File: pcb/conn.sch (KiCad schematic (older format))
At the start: 11 parts, among them P1 CONN_16X2, P2 CONN_16X2, P3 CONN_5X2

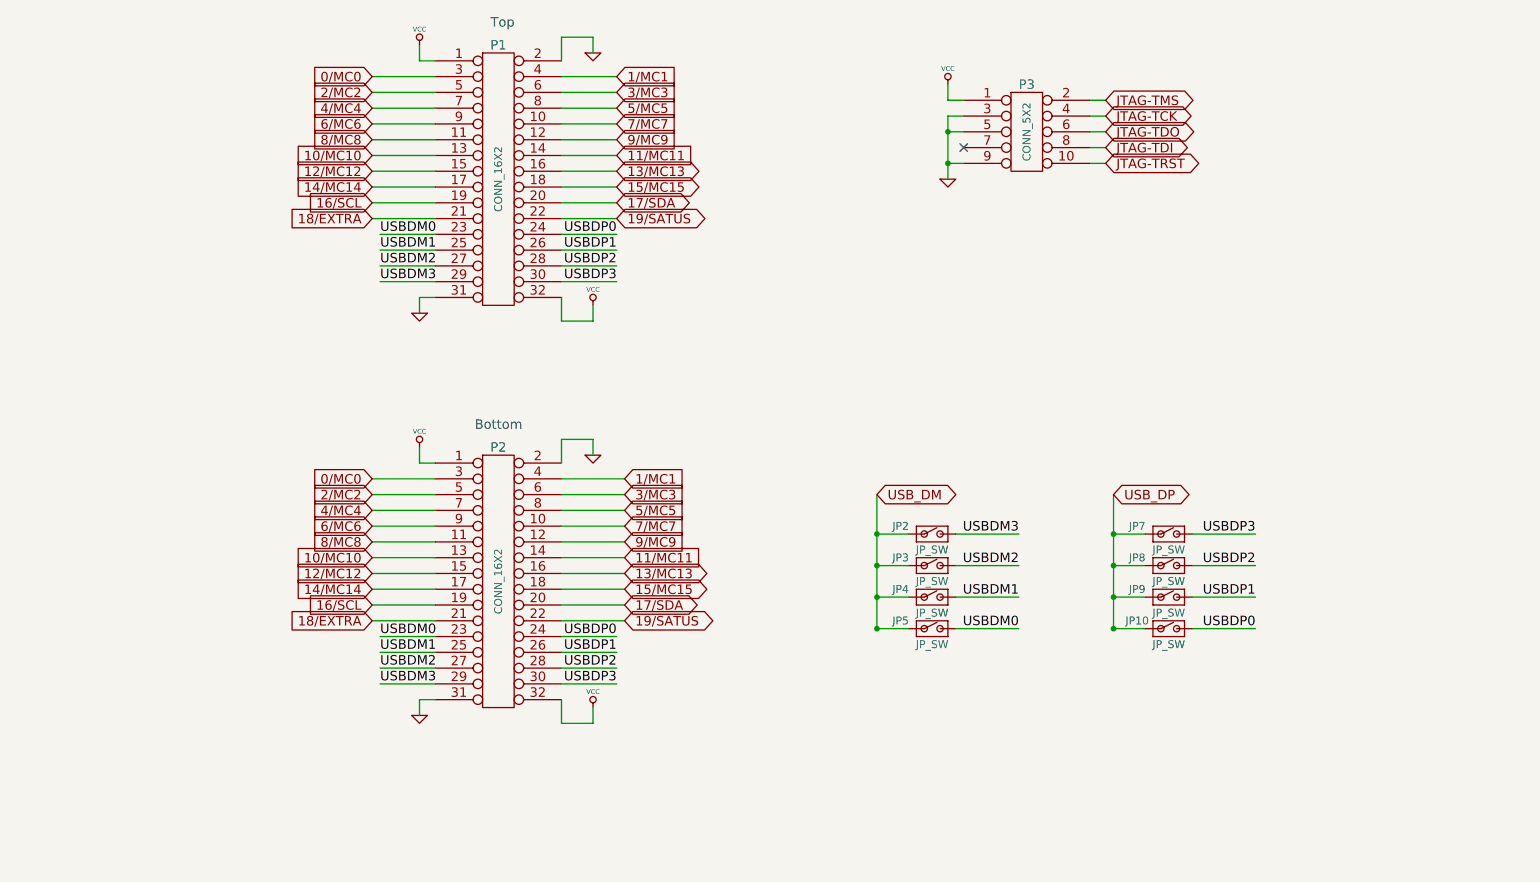
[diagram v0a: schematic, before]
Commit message: Work on single PCB version.
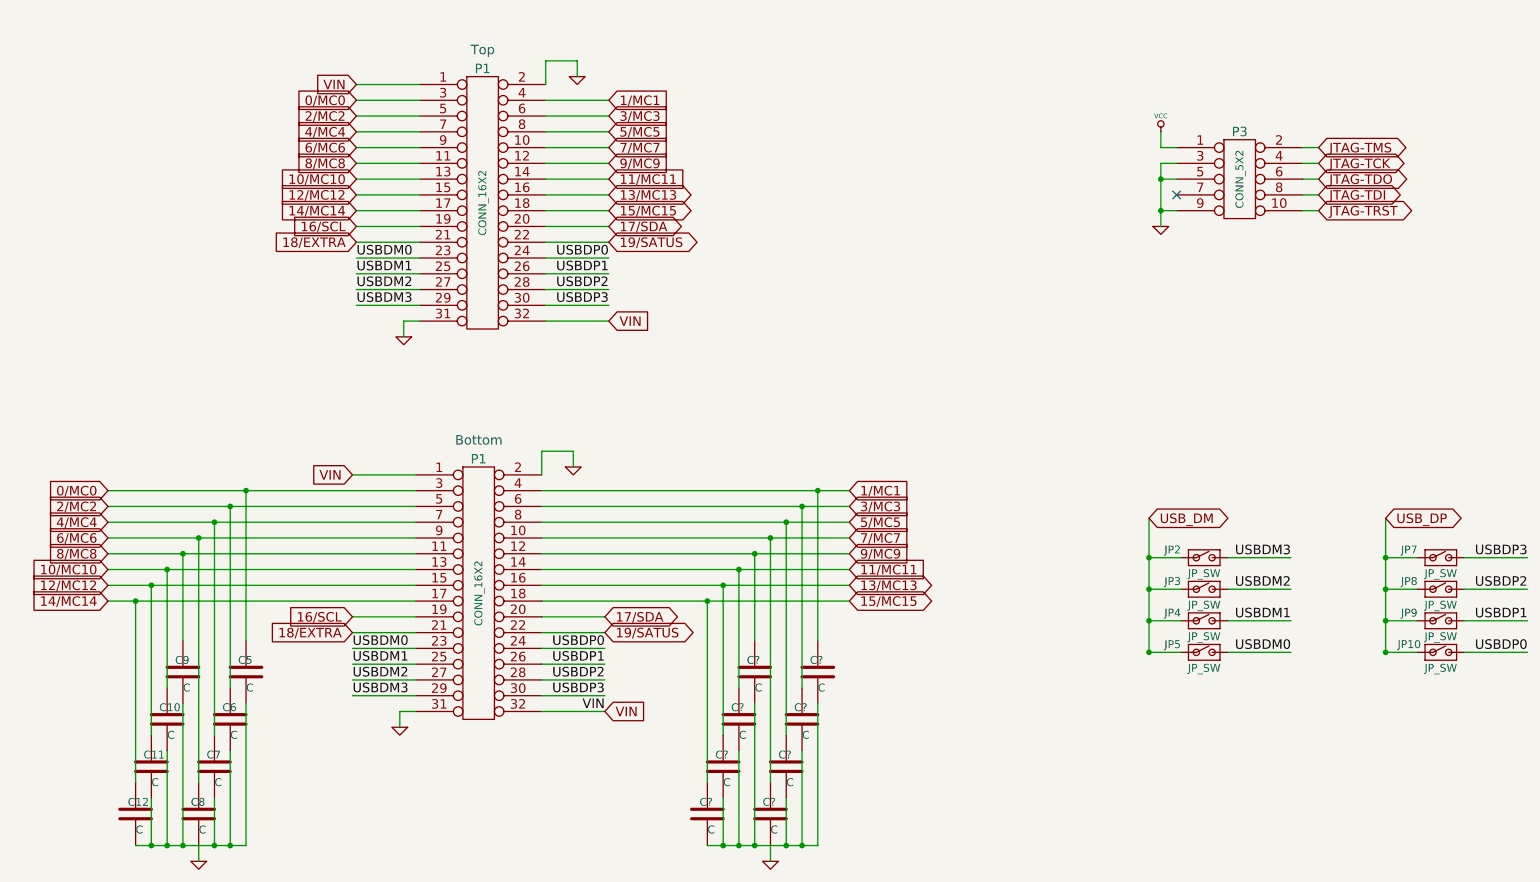
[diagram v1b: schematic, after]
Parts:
- removed P2: CONN_16X2, symbol CONN_16X2
- added C10, C11, C12, C5, C6, C7, C8, C9, C? (x8): C, symbol C
- added P1: CONN_16X2, symbol CONN_16X2
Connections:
- net 0/MC0: now also C5.1, P1.3 (P3)
- net 1/MC1: now also C?.1, P1.4 (P4)
- net 10/MC10: now also C10.1, P1.13 (P13)
- net 11/MC11: now also C?.1, P1.14 (P14)
- net 12/MC12: now also C11.1, P1.15 (P15)
- net 13/MC13: now also C?.1, P1.16 (P16)
- net 14/MC14: now also C12.1, P1.17 (P17)
- net 15/MC15: now also C?.1, P1.18 (P18)
- net 16/SCL: now also P1.19 (P19)
- net 17/SDA: now also P1.20 (P20)
- net 18/EXTRA: now also P1.21 (P21)
- net 19/SATUS: now also P1.22 (P22)
- net 2/MC2: now also C6.1, P1.5 (P5)
- net 3/MC3: now also C?.1, P1.6 (P6)
- net 4/MC4: now also C7.1, P1.7 (P7)
- net 5/MC5: now also C?.1, P1.8 (P8)
- net 6/MC6: now also C8.1, P1.9 (P9)
- net 7/MC7: now also C?.1, P1.10 (P10)
- net 8/MC8: now also C9.1, P1.11 (P11)
- net 9/MC9: now also C?.1, P1.12 (P12)
- net GND: now also C8.2, C?.2, P1.2 (P2), P1.31 (P31)
- net USBDM0: now also P1.23 (P23)
- net USBDM1: now also P1.25
- net USBDM2: now also P1.27 (P27)
- net USBDM3: now also P1.29 (P29)
- net USBDP0: now also P1.24 (P24)
- net USBDP1: now also P1.26 (P26)
- net USBDP2: now also P1.28 (P28)
- net USBDP3: now also P1.30 (P30)
- net VCC: no longer P1.1 (P1), P1.32 (P32)
- new net: C10.2, C11.2, C12.2, C5.2, C6.2, C7.2, C9.2
- new net: C?.2, C?.2, C?.2, C?.2, C?.2, C?.2, C?.2
- new net VIN: P1.1 (P1), P1.1 (P1), P1.32 (P32), P1.32 (P32)
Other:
- moved on the sheet: JP10, JP2, JP3, JP4, JP5, JP7, JP8, JP9, P1, P3
